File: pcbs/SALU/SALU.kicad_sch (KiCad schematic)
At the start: 0 parts

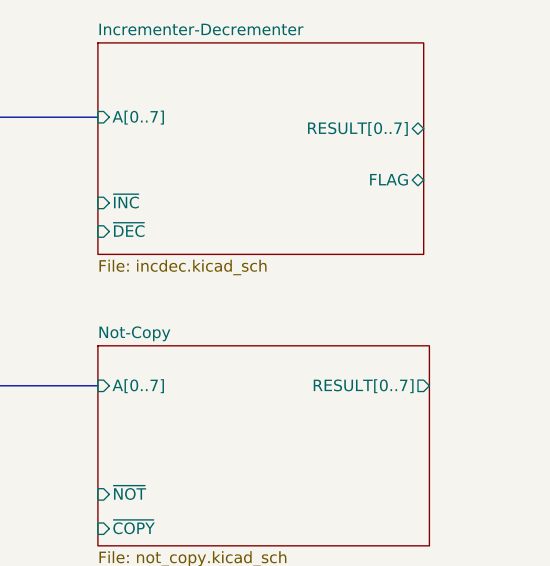
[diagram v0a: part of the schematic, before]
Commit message: Routing, routing, routing
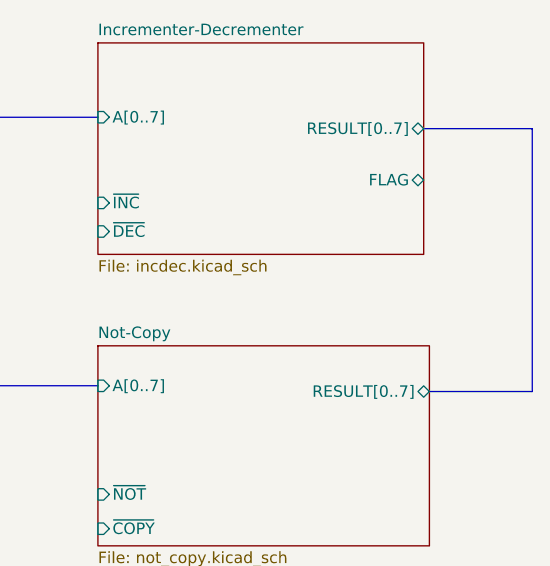
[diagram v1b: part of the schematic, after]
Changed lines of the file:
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@@
+    (stroke (width 0) (type default) (color 0 0 0 0))
+  )
+  (bus (pts (xy 197.485 58.42) (xy 186.055 58.42))
     (stroke (width 0) (type default) (color 0 0 0 0))
   )
@@
     (stroke (width 0) (type default) (color 0 0 0 0))
   )
+  (bus (pts (xy 197.485 29.21) (xy 197.485 58.42))
+    (stroke (width 0) (type default) (color 0 0 0 0))
+  )
   (bus (pts (xy 141.605 127) (xy 141.605 90.17))
+    (stroke (width 0) (type default) (color 0 0 0 0))
+  )
+  (bus (pts (xy 185.42 29.21) (xy 197.485 29.21))
     (stroke (width 0) (type default) (color 0 0 0 0))
   )
@@
       (effects (font (size 1.27 1.27)) (justify left))
     )
-    (pin "RESULT[0..7]" output (at 186.055 57.785 0)
+    (pin "RESULT[0..7]" tri_state (at 186.055 58.42 0)
       (effects (font (size 1.27 1.27)) (justify right))
     )

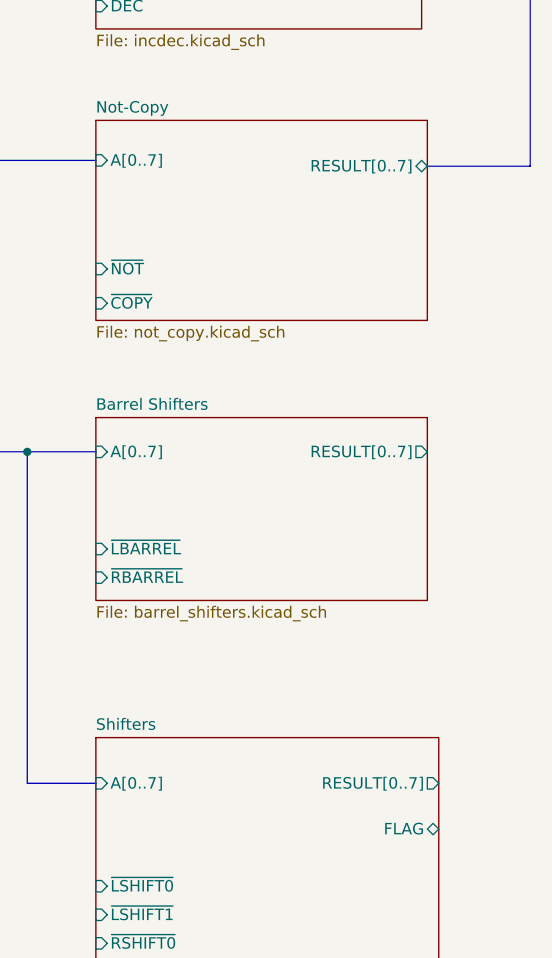
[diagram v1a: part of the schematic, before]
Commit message: More routing
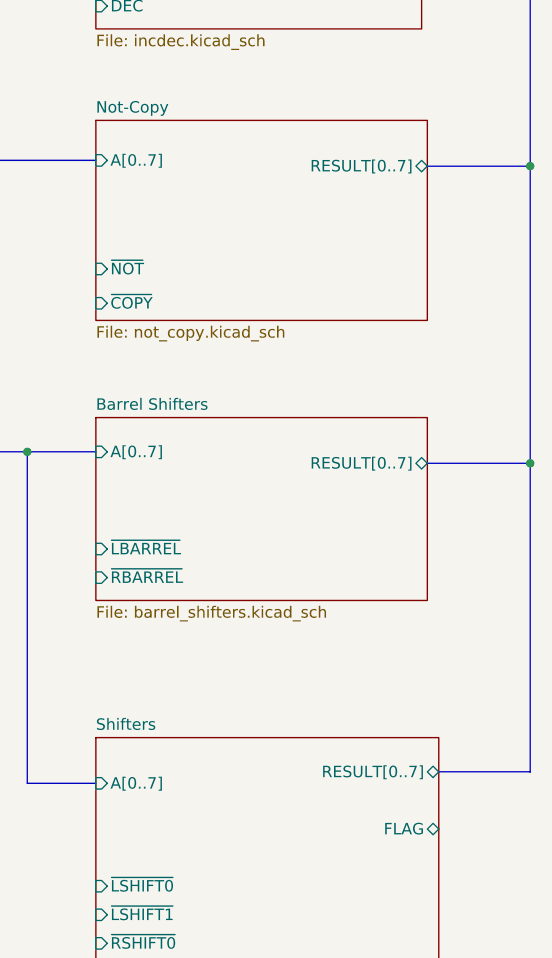
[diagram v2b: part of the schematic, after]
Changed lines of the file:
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@@
 (kicad_sch (version 20211123) (generator eeschema)
   (paper "A4")
+  (junction (at 197.485 91.44) (diameter 0) (color 0 0 0 0)
+  )
   (junction (at 107.95 57.785) (diameter 0) (color 0 0 0 0)
+  )
+  (junction (at 197.485 58.42) (diameter 0) (color 0 0 0 0)
   )
   (junction (at 141.605 90.17) (diameter 0) (color 0 0 0 0)
@@
   )
   (bus (pts (xy 107.95 57.785) (xy 107.95 49.53))
+    (stroke (width 0) (type default) (color 0 0 0 0))
+  )
+  (bus (pts (xy 197.485 125.73) (xy 187.325 125.73))
+    (stroke (width 0) (type default) (color 0 0 0 0))
+  )
+  (bus (pts (xy 186.055 91.44) (xy 197.485 91.44))
     (stroke (width 0) (type default) (color 0 0 0 0))
   )
@@
   )
   (bus (pts (xy 34.29 86.995) (xy 34.29 119.38))
+    (stroke (width 0) (type default) (color 0 0 0 0))
+  )
+  (bus (pts (xy 197.485 58.42) (xy 197.485 91.44))
     (stroke (width 0) (type default) (color 0 0 0 0))
   )
@@
   )
   (bus (pts (xy 81.28 69.215) (xy 91.44 69.215))
+    (stroke (width 0) (type default) (color 0 0 0 0))
+  )
+  (bus (pts (xy 197.485 91.44) (xy 197.485 125.73))
     (stroke (width 0) (type default) (color 0 0 0 0))
   )
@@
       (effects (font (size 1.27 1.27)) (justify left))
     )
-    (pin "RESULT[0..7]" output (at 186.055 90.17 0)
-      (effects (font (size 1.27 1.27)) (justify right))
-    )
     (pin "A[0..7]" input (at 149.225 90.17 180)
       (effects (font (size 1.27 1.27)) (justify left))
+    )
+    (pin "RESULT[0..7]" tri_state (at 186.055 91.44 0)
+      (effects (font (size 1.27 1.27)) (justify right))
     )
   )
@@
       (effects (font (size 1.27 1.27)) (justify left))
     )
-    (pin "RESULT[0..7]" output (at 187.325 127 0)
-      (effects (font (size 1.27 1.27)) (justify right))
-    )
     (pin "~{RSHIFT0}" input (at 149.225 144.78 180)
       (effects (font (size 1.27 1.27)) (justify left))
@@
       (effects (font (size 1.27 1.27)) (justify right))
     )
+    (pin "RESULT[0..7]" tri_state (at 187.325 125.73 0)
+      (effects (font (size 1.27 1.27)) (justify right))
+    )
